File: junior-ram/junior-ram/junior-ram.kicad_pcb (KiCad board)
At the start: 2 copper layers, 160 x 100 mm, 7 parts, among them IC1 74LS241, IC2 74LS241, IC3 74LS243, IC4 74LS243, IC5 GAL16V8, J1 C64AC

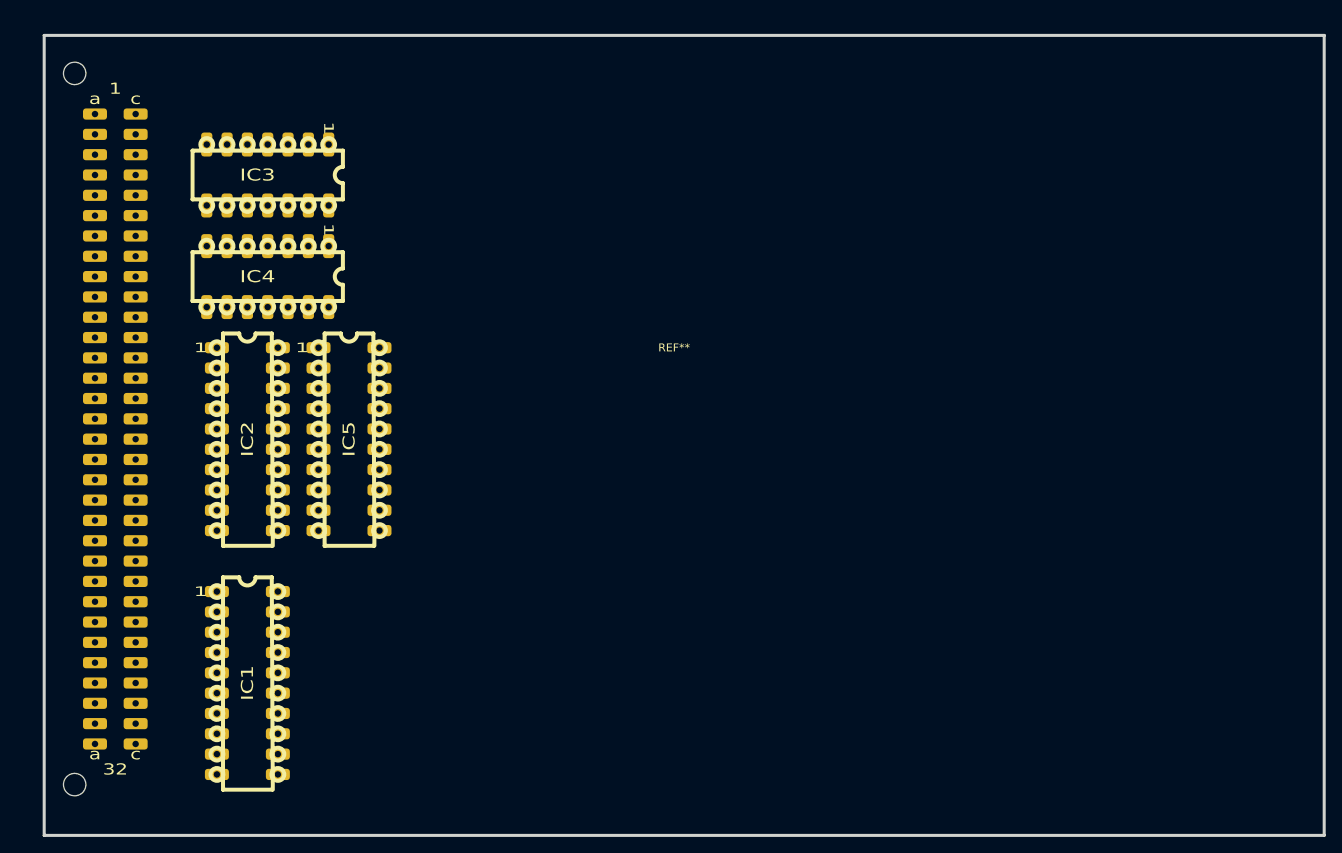
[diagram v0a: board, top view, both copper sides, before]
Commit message: junior ram
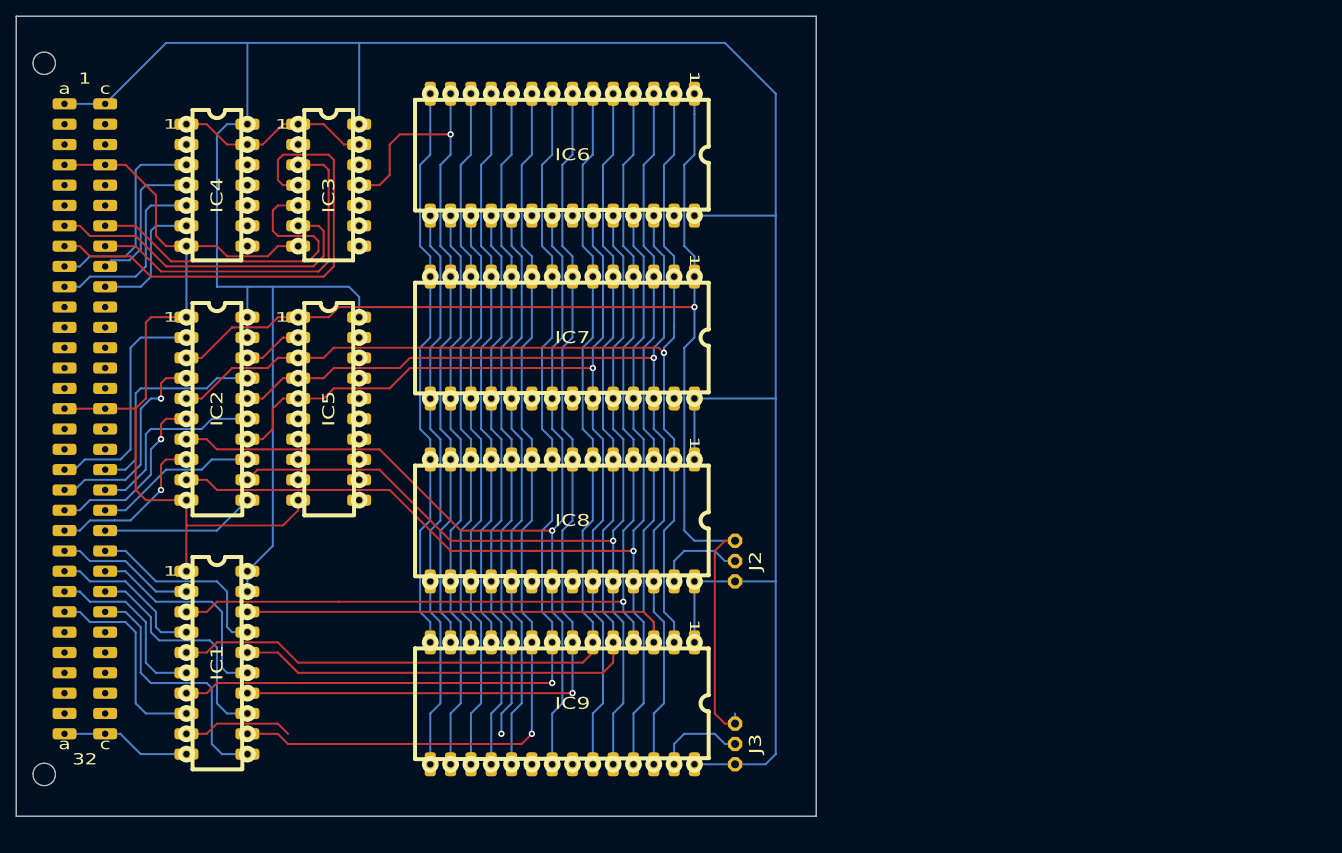
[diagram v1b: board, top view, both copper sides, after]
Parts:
- removed REF**: EuroBoard160mmX100mm, EuroBoard_Outline:EuroBoard160mmX100mm
- added IC6: 62256, elektor:DIL-28, F.Cu at (130.8, 67.3)
- added IC7: 62256, elektor:DIL-28, F.Cu at (130.8, 90.2)
- added IC8: 27C256, elektor:DIL-28, F.Cu at (130.8, 113.0)
- added IC9: 27C256, elektor:DIL-28, F.Cu at (130.8, 135.9)
- added J2: Conn_01x03_Male, elektor:CONN-3, F.Cu at (149.9, 118.1)
- added J3: Conn_01x03_Male, elektor:CONN-3, F.Cu at (149.9, 141.0)
- moved IC4 13.1 mm to (85.1, 71.1), turned to 270 degrees
- moved IC3 7.73 mm to (99.1, 71.1), turned to 270 degrees
- moved IC2 5.39 mm to (85.1, 97.8)
- moved IC1 4.58 mm to (85.1, 129.5)
- moved IC5 4.58 mm to (99.1, 97.8)
- moved J1 4.02 mm to (68.6, 61.0)
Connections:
- IC5 pad 1: AB11 -> AB14
- IC5 pad 2: AB12 -> AB15
- IC5 pad 3: AB13 -> AB12
- IC5 pad 4: AB14 -> AB13
- IC5 pad 5: AB15 -> AB11
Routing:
- net +5V: track 0.00 -> 344.0 mm
- net GND: track 0.00 -> 201.9 mm
- net AB14: track 0.00 -> 156.9 mm, vias 0 -> 1
- net AB12: track 0.00 -> 134.3 mm, vias 0 -> 1
- net AB8: track 0.00 -> 131.3 mm, vias 0 -> 1
- net AB6: track 0.00 -> 126.9 mm, vias 0 -> 1
- net AB4: track 0.00 -> 125.9 mm
- net AB7: track 0.00 -> 125.6 mm
- net AB13: track 0.00 -> 124.6 mm, vias 0 -> 1
- net AB2: track 0.00 -> 123.1 mm, vias 0 -> 1
- net AB10: track 0.00 -> 122.2 mm, vias 0 -> 1
- net AB9: track 0.00 -> 121.7 mm, vias 0 -> 1
- net AB5: track 0.00 -> 121.6 mm
- net AB11: track 0.00 -> 120.1 mm, vias 0 -> 1
- net AB1: track 0.00 -> 119.8 mm, vias 0 -> 1
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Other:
- board size 160 x 100 mm -> 100 x 100 mm
